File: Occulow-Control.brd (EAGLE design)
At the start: 38.1 x 104.1 mm, 46 parts, among them T1 DMP3010LK3, T2 DMP3010LK3, T3 DMP3010LK3

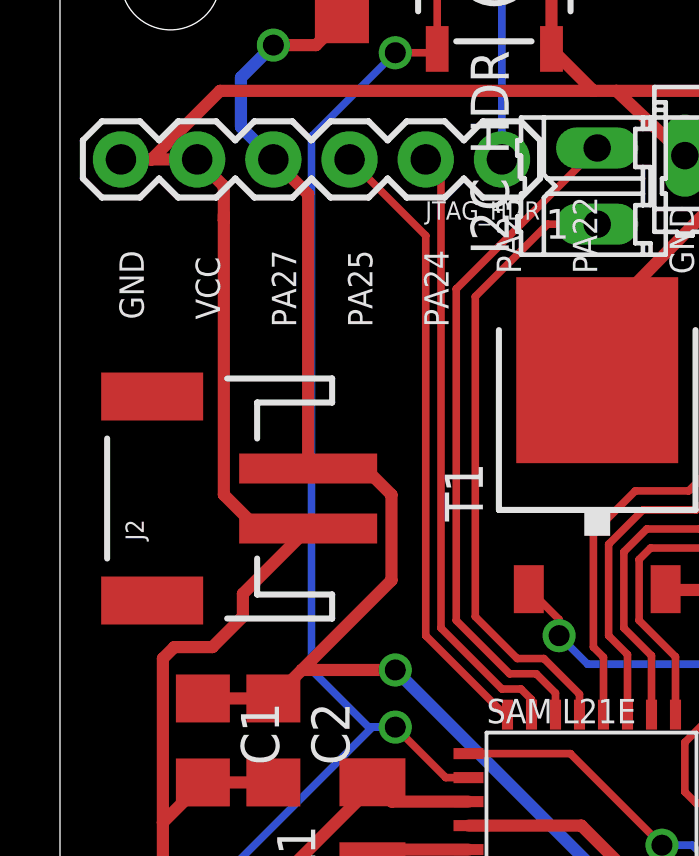
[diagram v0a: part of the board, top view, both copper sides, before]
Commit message: Created 2 wire trap lib, placed in schematic
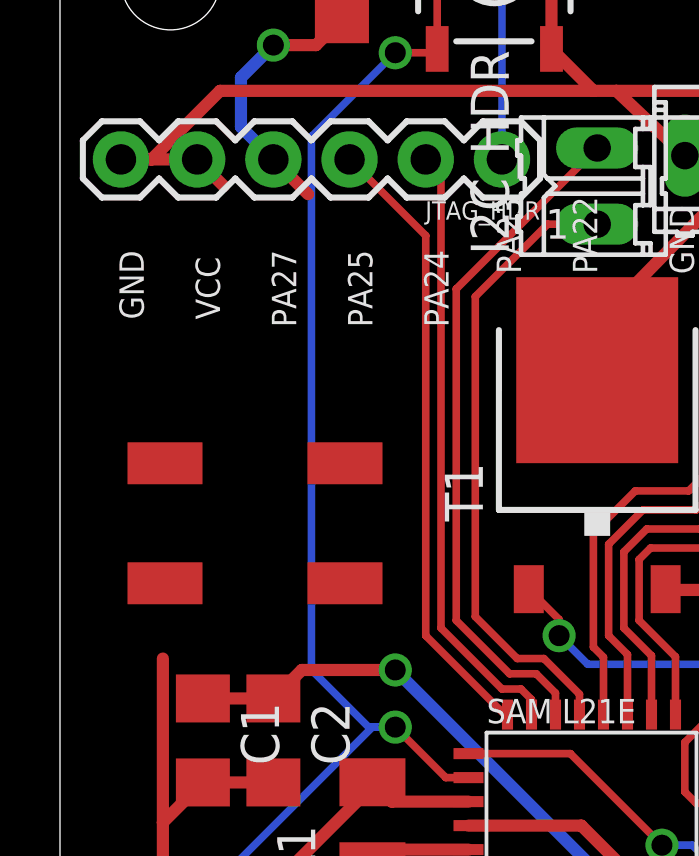
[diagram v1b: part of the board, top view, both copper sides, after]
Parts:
- removed J2: (no value), SparkFun-Connectors:JST-2-SMD
- added U$7: MINI-LITE-TRAP, lite-trap:MINI-LITE-TRAP
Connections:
- net GND: now also U$7.3, U$7.4; no longer J2.1
- net VCC: now also U$7.1, U$7.2; no longer J2.2
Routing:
- net GND: track 170.5 -> 149.6 mm
- net VCC: track 107.9 -> 88.5 mm
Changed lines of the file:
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@@
 <?xml version="1.0" encoding="utf-8"?>
 <!DOCTYPE eagle SYSTEM "eagle.dtd">
-<eagle version="8.0.2">
+<eagle version="8.1.0">
 <drawing>
 <settings>
@@
 <setting verticaltext="up"/>
 </settings>
-<grid distance="0.01" unitdist="inch" unit="inch" style="lines" multiple="1" display="no" altdistance="0.005" altunitdist="inch" altunit="inch"/>
+<grid distance="1" unitdist="mm" unit="mm" style="lines" multiple="1" display="no" altdistance="0.05" altunitdist="mm" altunit="mm"/>
 <layers>
 <layer number="1" name="Top" color="4" fill="1" visible="yes" active="yes"/>
@@
 <attribute name="OC_NEWARK" value="unknown" x="34.7345" y="26.4795" size="1.778" layer="27" rot="R90" display="off"/>
 </element>
-<element name="J2" library="SparkFun-Connectors" package="JST-2-SMD" value="" x="4.572" y="28.575" rot="R90">
-<attribute name="PROD_ID" value="CONN-11443" x="4.572" y="28.575" size="1.778" layer="27" rot="R90" display="off"/>
-<attribute name="SF_ID" value="PRT-08612" x="4.572" y="28.575" size="1.778" layer="27" rot="R90" display="off"/>
-</element>
 <element name="L1" library="resistor" package="L3225M" value="10uH" x="10.414" y="17.7165" rot="R90"/>
 <element name="L2" library="SparkFun-Coils" package="0603" value="" x="28.1305" y="10.4775" rot="R270">
@@
 <attribute name="OC_NEWARK" value="unknown" x="17.907" y="38.989" size="1.778" layer="27" rot="R90" display="off"/>
 </element>
+<element name="U$7" library="lite-trap" package="MINI-LITE-TRAP" value="MINI-LITE-TRAP" x="6.5" y="28.25"/>
 </elements>
 <signals>
@@
 <contactref element="GRIDEYE_HDR" pad="5"/>
 <contactref element="PIR_HDR" pad="2"/>
-<contactref element="J2" pad="1"/>
 <contactref element="C7" pad="2"/>
 <contactref element="C1" pad="2"/>
@@
 <wire x1="3.429" y1="17.777" x2="4.7625" y2="19.1105" width="0.4064" layer="1"/>
 <wire x1="3.429" y1="17.777" x2="3.429" y2="23.241" width="0.4064" layer="1"/>
-<wire x1="3.429" y1="23.241" x2="3.81" y2="23.622" width="0.4064" layer="1"/>
-<wire x1="3.81" y1="23.622" x2="5.08" y2="23.622" width="0.4064" layer="1"/>
-<wire x1="5.08" y1="23.622" x2="6.096" y2="24.638" width="0.4064" layer="1"/>
-<wire x1="6.096" y1="24.638" x2="6.096" y2="25.399" width="0.4064" layer="1"/>
-<wire x1="6.096" y1="25.399" x2="8.272" y2="27.575" width="0.4064" layer="1"/>
-<wire x1="8.272" y1="27.575" x2="6.588" y2="27.575" width="0.4064" layer="1"/>
-<wire x1="6.588" y1="27.575" x2="5.461" y2="28.702" width="0.4064" layer="1"/>
 <wire x1="20.828" y1="40.005" x2="18.542" y2="42.164" width="0.4064" layer="1"/>
 <wire x1="3.429" y1="13.335" x2="3.429" y2="12.827" width="0.4064" layer="1"/>
@@
 <wire x1="23.368" y1="15.24" x2="21.8485" y2="15.24" width="0.4064" layer="1"/>
 <wire x1="21.8485" y1="15.24" x2="21.8165" y2="15.272" width="0.4064" layer="1"/>
-<wire x1="5.461" y1="28.702" x2="5.461" y2="37.846" width="0.4064" layer="1"/>
-<wire x1="5.461" y1="37.846" x2="5.461" y2="38.0365" width="0.4064" layer="1"/>
 <contactref element="S1" pad="3"/>
 <contactref element="S1" pad="4"/>
@@
 <contactref element="JTAG_HDR" pad="6"/>
 <contactref element="JTAG_HDR" pad="5"/>
-<wire x1="5.461" y1="37.846" x2="5.461" y2="38.989" width="0.4064" layer="1"/>
 <wire x1="5.461" y1="38.989" x2="4.572" y2="39.878" width="0.4064" layer="1"/>
 <wire x1="3.048" y1="39.878" x2="4.572" y2="39.878" width="0.4064" layer="1"/>
@@
 <wire x1="5.334" y1="42.164" x2="3.048" y2="39.878" width="0.4064" layer="1"/>
 <wire x1="17.78" y1="42.164" x2="5.334" y2="42.164" width="0.4064" layer="1"/>
+<contactref element="U$7" pad="4"/>
+<contactref element="U$7" pad="3"/>
+<wire x1="3.5" y1="25.75" x2="5.461" y2="38.989" width="0" layer="19" extent="1-1"/>
+<wire x1="3.429" y1="23.241" x2="3.5" y2="25.75" width="0" layer="19" extent="1-1"/>
+<wire x1="9.5" y1="25.75" x2="3.429" y2="23.241" width="0" layer="19" extent="1-1"/>
 </signal>
 <signal name="VCC">
-<contactref element="J2" pad="2"/>
 <contactref element="L2" pad="2"/>
 <contactref element="C1" pad="1"/>
@@
 <wire x1="29.464" y1="10.795" x2="29.464" y2="16.605" width="0.4064" layer="1"/>
 <wire x1="30.994" y1="18.135" x2="29.464" y2="16.605" width="0.4064" layer="1"/>
-<wire x1="10.176" y1="29.575" x2="8.272" y2="29.575" width="0.4064" layer="1"/>
-<wire x1="10.176" y1="29.575" x2="11.049" y2="28.702" width="0.4064" layer="1"/>
-<wire x1="11.049" y1="28.702" x2="11.049" y2="25.8475" width="0.4064" layer="1"/>
-<wire x1="8.0615" y1="22.86" x2="11.049" y2="25.8475" width="0.4064" layer="1"/>
 <wire x1="8.0615" y1="22.86" x2="7.112" y2="21.9105" width="0.4064" layer="1"/>
 <wire x1="13.6165" y1="16.072" x2="12.897" y2="16.072" width="0.4064" layer="1"/>
@@
 <contactref element="JTAG_HDR" pad="4"/>
 <wire x1="8.272" y1="38.718" x2="7.112" y2="39.878" width="0.4064" layer="1"/>
-<wire x1="8.272" y1="29.575" x2="8.272" y2="38.718" width="0.4064" layer="1"/>
 <wire x1="6.0325" y1="42.6085" x2="6.0325" y2="40.9575" width="0.4064" layer="16"/>
 <wire x1="6.0325" y1="40.9575" x2="7.112" y2="39.878" width="0.4064" layer="16"/>
+<contactref element="U$7" pad="1"/>
+<contactref element="U$7" pad="2"/>
+<wire x1="9.5" y1="29.75" x2="8.272" y2="38.718" width="0" layer="19" extent="1-1"/>
+<wire x1="3.5" y1="29.75" x2="9.5" y2="29.75" width="0" layer="19" extent="1-1"/>
+<wire x1="8.0615" y1="22.86" x2="9.5" y2="29.75" width="0" layer="19" extent="1-1"/>
 </signal>
 <signal name="RF">
